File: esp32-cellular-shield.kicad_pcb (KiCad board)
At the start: 2 copper layers, 68.5 x 53.3 mm, 63 parts, among them J2 CONN_01X05, Q1 Q_NPN_BEC, Q2 Q_NPN_BEC, Q3 Q_NPN_BEC, Q4 AO3401_PMOS_GSD, SW1 SW_Push, U1 SIM_HOLDER, U2 SIM800C, U3 Ra-02, U4 MCP601OT, U6 MCP16311-MNY, U7 TC1264-3.3VAB

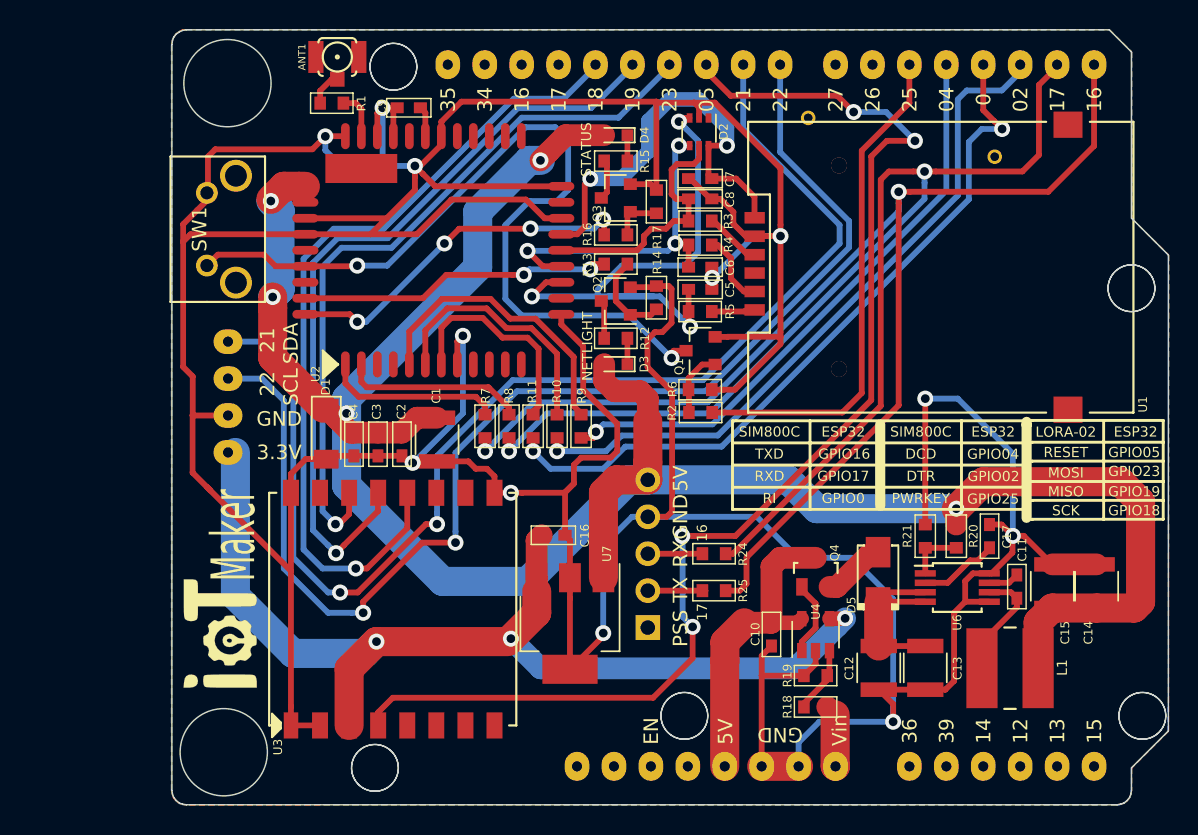
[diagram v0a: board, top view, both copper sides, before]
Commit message: drop IC PWR 3.3V & swap pin connect to the module
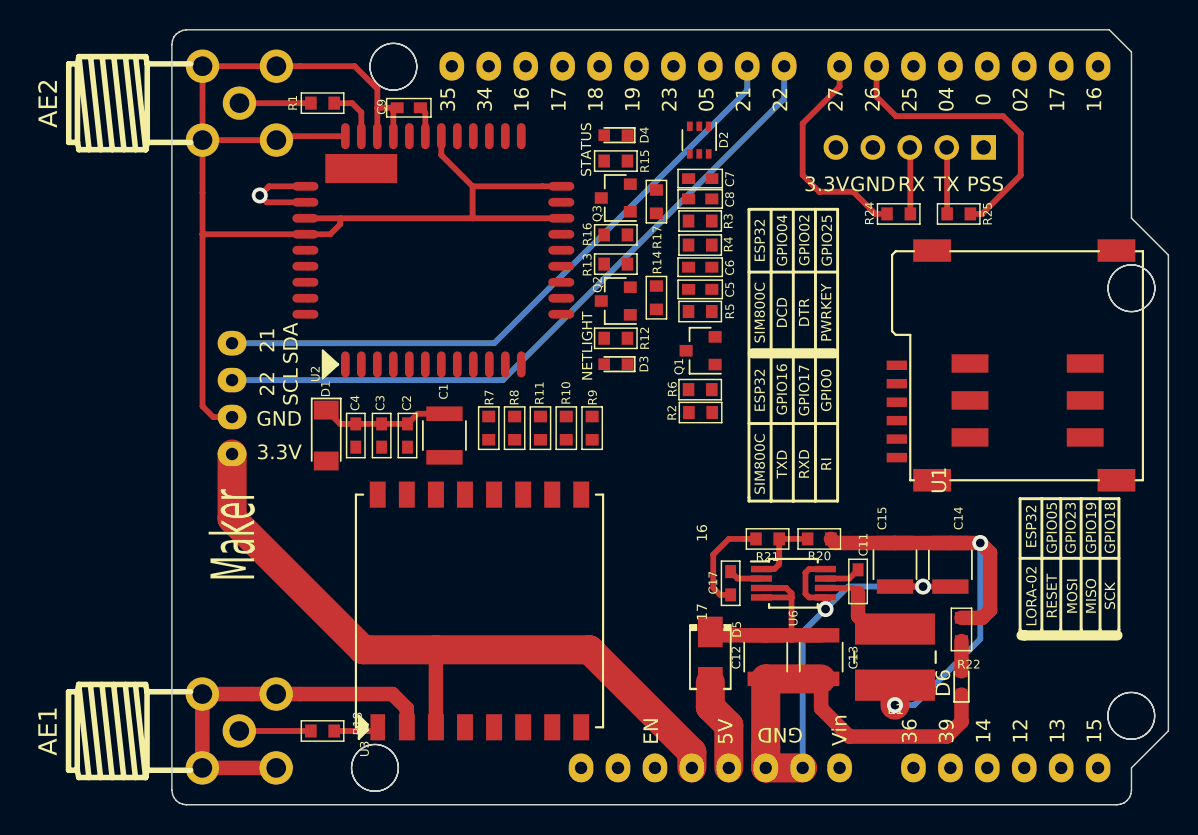
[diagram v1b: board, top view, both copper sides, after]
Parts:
- removed ANT1: ANTENNA, lib:coaxial_u.fl-r-smt-1
- removed C10: 100nF, lib:C_0603
- removed C16: 1uF/25V, lib:C_0603
- removed G***: LOGO, lib:logo-iotmakervn_7.5x5
- removed Q4: AO3401_PMOS_GSD, lib:SOT-23
- removed R19: 10k, lib:R_0603
- removed REF** (x2): SolderWirePad_single_1mmDrill, Wire_Pads:SolderWirePad_single_1mmDrill
- removed SW1: SW_Push, lib:Tact_switch-4pin
- removed U4: MCP601OT, TO_SOT_Packages_SMD:SOT-23-5
- removed U7: TC1264-3.3VAB, TO_SOT_Packages_SMD:SOT-223-3Lead_TabPin2
- added AE1: Antenna_Shield, lib:sma_90_r300.124.403, F.Cu at (109.4, 99.1)
- added AE2: Antenna_Shield, lib:sma_90_r300.124.403, F.Cu at (109.4, 55.9)
- added D6: Led_PWR, LEDs:LED_0603, F.Cu at (163.3, 95.8)
- added R22: 470R, lib:R_0603, F.Cu at (163.3, 92.1)
- J2: footprint Pin_Headers:Pin_Header_Straight_1x05_Pitch2.54mm -> lib:Pin_Header_NEO6M_GPS_R2_1x05_Pitch2.54mm
- R18: value 10k -> 0R
- R20: value 200k/1% -> 52.5k/1%
- R21: value 47k/1% -> 12k/1%
- U1: footprint lib:sim_socket_PP -> lib:MicroSim-Socket-6P
- moved J2 40.3 mm to (164.8, 58.9), turned to 270 degrees
- moved R18 33.9 mm to (119.4, 99.1)
- moved R25 30.9 mm to (163.1, 63.5)
- moved R24 26.6 mm to (159.0, 63.5), turned to 180 degrees
- moved C17 18.1 mm to (147.4, 88.9), turned to 270 degrees
- moved U1 17.4 mm to (161.3, 81.8), turned to 90 degrees
- moved D5 12.8 mm to (146.1, 94.0), turned to 90 degrees
- moved U6 11.3 mm to (151.8, 88.9)
- moved C11 10.9 mm to (156.2, 88.8)
- moved C15 10.9 mm to (158.8, 87.6), turned to 270 degrees
- moved R21 10.8 mm to (150.0, 85.9), turned to 180 degrees
- moved C14 10.2 mm to (162.6, 87.6), turned to 270 degrees
- moved R20 9.43 mm to (153.5, 85.9), turned to 180 degrees
- moved L1 7.95 mm to (158.8, 94.0), turned to 270 degrees
- moved C12 7.81 mm to (149.9, 94.0)
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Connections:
- D2 pad 1: (no net) -> Net-(D2-Pad1)
- D5 pad 2: +5V -> +5VD
- J2 pad 1: (no net) -> Net-(J2-Pad1)
- J2 pad 5: VDD -> +3V3
- R1 pad 1: GSM_ANT -> Net-(AE2-Pad1)
- R1 pad 2: Net-(ANT1-Pad1) -> Net-(R1-Pad2)
- R18 pad 2: Vin -> Net-(R18-Pad2)
- R7 pad 1: GPS_TX -> SIM800C_TXD
- R8 pad 1: GPS_RX -> SIM800C_RXD
- S1 pad 1: (no net) -> Net-(S1-Pad1)
- S1 pad 10: (no net) -> RA_CS
- S1 pad 11: (no net) -> RA_SCK
- S1 pad 12: (no net) -> RA_MISO/SPIQ
- S1 pad 13: (no net) -> RA_MOSI/SPID
- S1 pad 14: (no net) -> RA_RESET
- S1 pad 15: GPS_TX -> Net-(S1-Pad15)
- S1 pad 16: GPS_RX -> Net-(S1-Pad16)
- S1 pad 17: SIM800C_DTR -> Net-(S1-Pad17)
- S1 pad 18: SIM800C_RI -> Net-(S1-Pad18)
- S1 pad 19: SIM800C_DCD -> Net-(S1-Pad19)
- S1 pad 2: (no net) -> Net-(S1-Pad2)
- S1 pad 20: PWRKEY -> Net-(S1-Pad20)
- S1 pad 21: (no net) -> GPS_TX
- S1 pad 22: (no net) -> GPS_RX
- S1 pad 25: RA_RESET -> SIM800C_DTR
- S1 pad 26: RA_MOSI/SPID -> SIM800C_RI
- S1 pad 27: RA_MISO/SPIQ -> SIM800C_DCD
- S1 pad 28: RA_SCK -> PWRKEY
- S1 pad 29: (no net) -> SIM800C_RXD
- S1 pad 3: (no net) -> Net-(S1-Pad3)
- S1 pad 30: (no net) -> SIM800C_TXD
- S1 pad 31: (no net) -> Net-(S1-Pad31)
- S1 pad 32: (no net) -> Net-(S1-Pad32)
- S1 pad 4: (no net) -> +3V3
- S1 pad 9: (no net) -> Net-(S1-Pad9)
- U1 pad 6: (no net) -> Net-(U1-Pad6)
- U2 pad 10: (no net) -> Net-(U2-Pad10)
- U2 pad 11: (no net) -> Net-(U2-Pad11)
- U2 pad 12: (no net) -> Net-(U2-Pad12)
- U2 pad 14: (no net) -> Net-(U2-Pad14)
- U2 pad 20: (no net) -> Net-(U2-Pad20)
- U2 pad 22: (no net) -> UART2_T
- U2 pad 23: (no net) -> UART2_R
- U2 pad 24: (no net) -> USB_VBUS
- U2 pad 25: (no net) -> USB_DP
- U2 pad 26: (no net) -> Net-(U2-Pad26)
- U2 pad 29: (no net) -> Net-(U2-Pad29)
- U2 pad 3: (no net) -> Net-(U2-Pad3)
- U2 pad 32: GSM_ANT -> Net-(R1-Pad2)
- U2 pad 38: (no net) -> ADC
- U2 pad 4: (no net) -> Net-(U2-Pad4)
- U2 pad 40: (no net) -> Net-(U2-Pad40)
- U2 pad 9: (no net) -> Net-(U2-Pad9)
- U3 pad 1: GND -> Net-(R18-Pad2)
- U3 pad 10: (no net) -> Net-(U3-Pad10)
- U3 pad 11: (no net) -> Net-(U3-Pad11)
- U3 pad 15: (no net) -> RA_CS
- U3 pad 5: (no net) -> Net-(U3-Pad5)
- U3 pad 6: (no net) -> Net-(U3-Pad6)
- U3 pad 7: (no net) -> Net-(U3-Pad7)
- U3 pad 8: (no net) -> Net-(U3-Pad8)
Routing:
- net GND: track 414.9 -> 184.6 mm, vias 12 -> 2
- net VDD: track 167.8 -> 48.7 mm, vias 5 -> 3
- net RA_RESET: track 86.6 -> 0.00 mm, vias 4 -> 0
- net GPS_RX: track 87.3 -> 15.5 mm, vias 2 -> 0
- net GPS_TX: track 91.2 -> 20.5 mm, vias 2 -> 0
- net SIM800C_PWRKEY: track 58.2 -> 0.00 mm, vias 2 -> 0
- net RA_SCK: track 56.9 -> 0.00 mm, vias 1 -> 0
- net RA_MISO/SPIQ: track 53.7 -> 0.00 mm, vias 1 -> 0
- net SIM800C_RI: track 50.6 -> 0.00 mm, vias 2 -> 0
- net RA_MOSI/SPID: track 50.5 -> 0.00 mm, vias 1 -> 0
- net SIM800C_DTR: track 47.9 -> 0.00 mm, vias 1 -> 0
- net SIM800C_DCD: track 41.0 -> 0.00 mm, vias 1 -> 0
- net SDA: track 83.9 -> 44.3 mm, vias 2 -> 0
- net SIM800C_DATA: track 38.7 -> 0.00 mm, vias 3 -> 0
- net SCL: track 84.7 -> 48.2 mm, vias 2 -> 0
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- removed copper zone on B.Cu, net GND
- removed copper zone on F.Cu, net GND
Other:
- outline, holes or cut-outs redrawn
- net class Default: clearance 0.254 -> 0.1
- rule trace_clearance: 0.254 -> 0.1
